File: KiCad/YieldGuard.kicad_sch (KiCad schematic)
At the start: 3 parts, among them J1 Conn_01x04_Socket, U1 ESP32-DEVKITC, U2 HX711

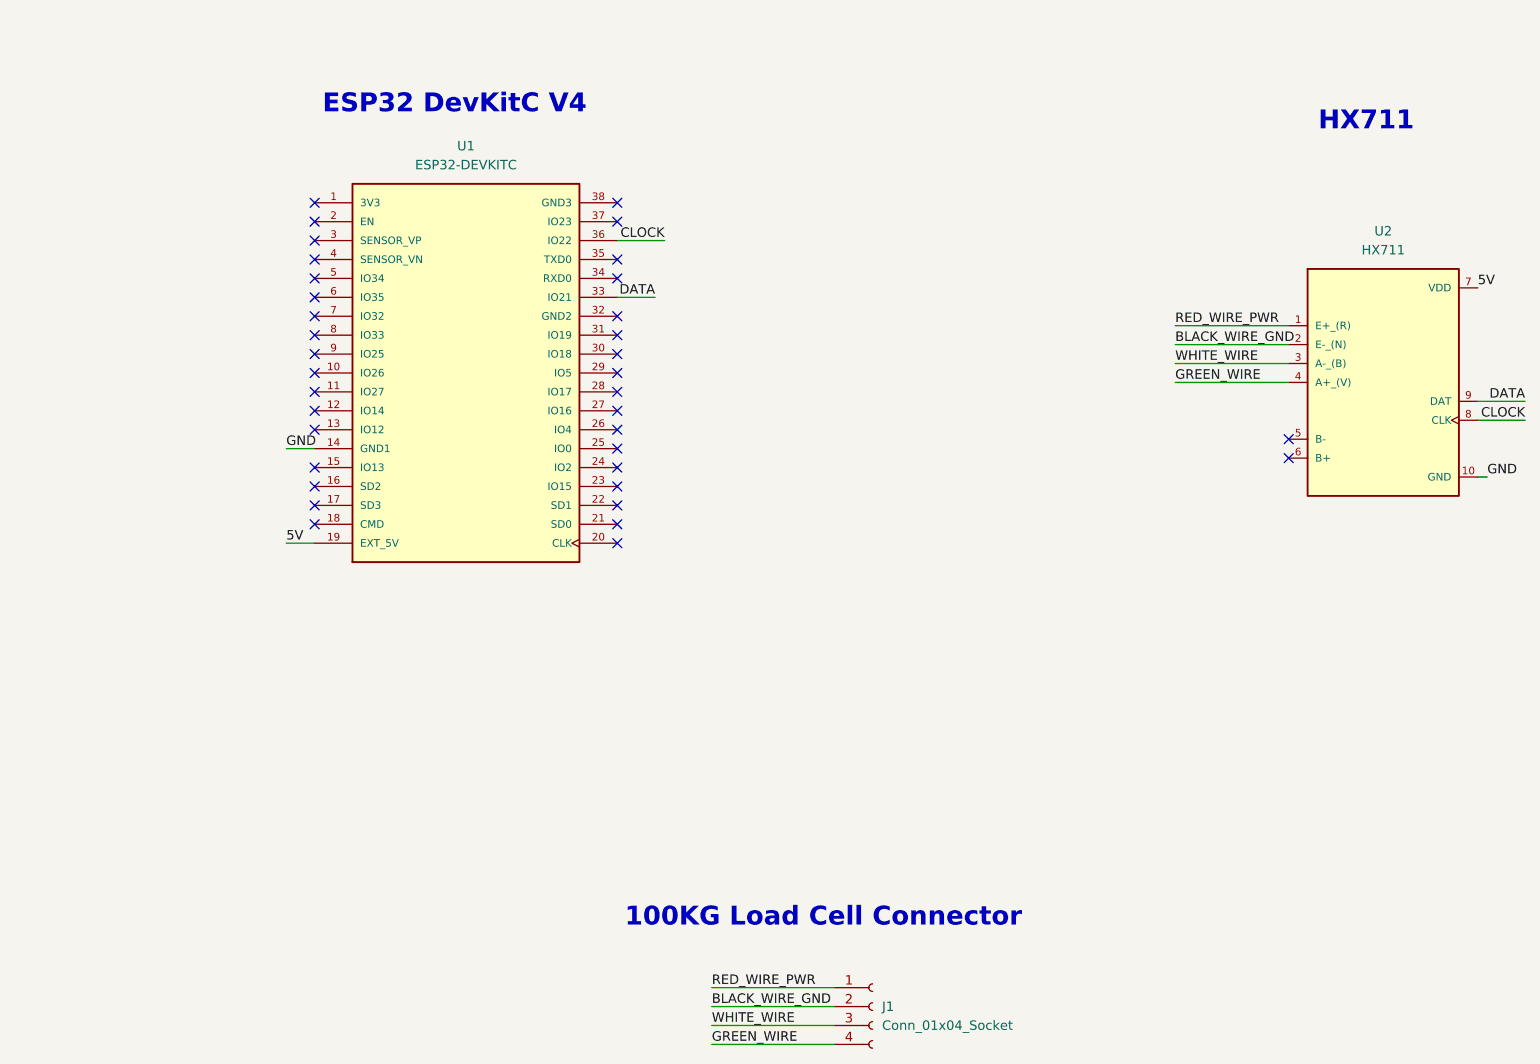
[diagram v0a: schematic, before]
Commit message: Bit changes in PCB and Schematic and Completed BoM
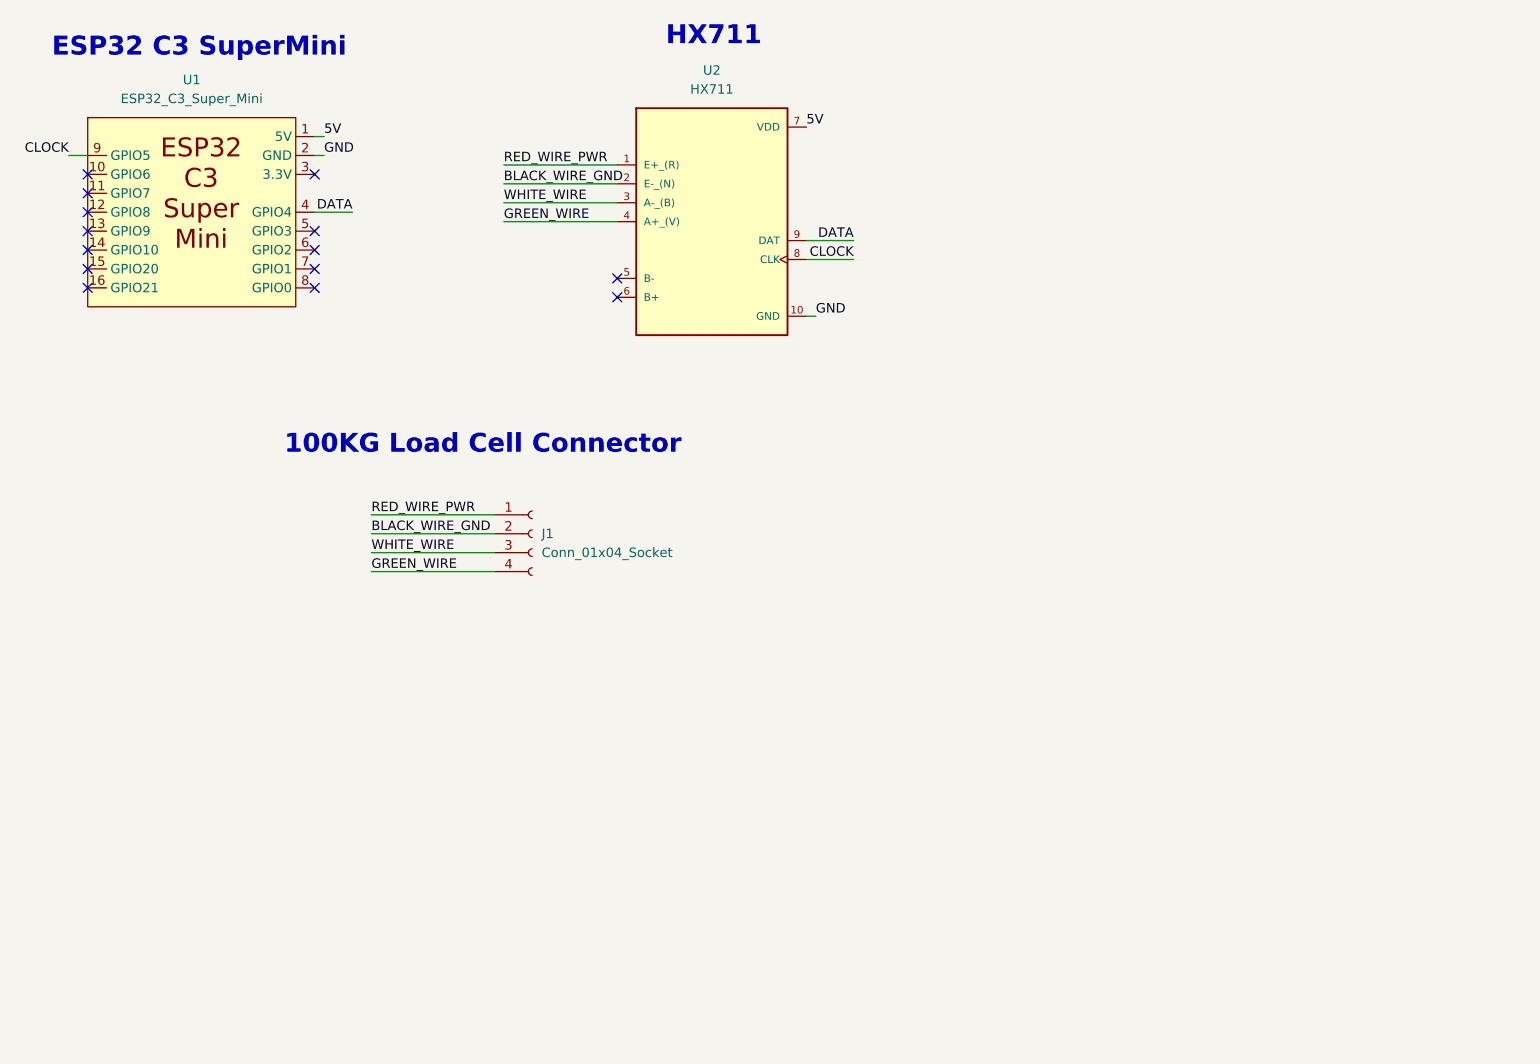
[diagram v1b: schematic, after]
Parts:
- removed U1: ESP32-DEVKITC, KiCad:MODULE_ESP32-DEVKITC, symbol ESP32-DEVKITC:ESP32-DEVKITC
- added U1: ESP32_C3_Super_Mini, KiCad:ESP32-C3_SuperMini, symbol ESP32-C3-SuperMini:ESP32_C2_Super_Mini
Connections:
- net 5V: now also U1.1 (5V)
- net CLOCK: now also U1.9 (GPIO5)
- net DATA: now also U1.4 (GPIO4)
- net GND: now also U1.2 (GND)
- no-connect marks 36 -> 14
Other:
- note added: "ESP32 C3 SuperMini"
- note removed: "ESP32 DevKitC V4"
- moved on the sheet: J1, U2
